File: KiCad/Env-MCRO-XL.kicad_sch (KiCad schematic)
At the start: 74 parts, among them SW1 RotaryEncoder_Switch, SW2 RotaryEncoder_Switch, SW3 RotaryEncoder_Switch, SW4 RotaryEncoder_Switch, U1 Pico

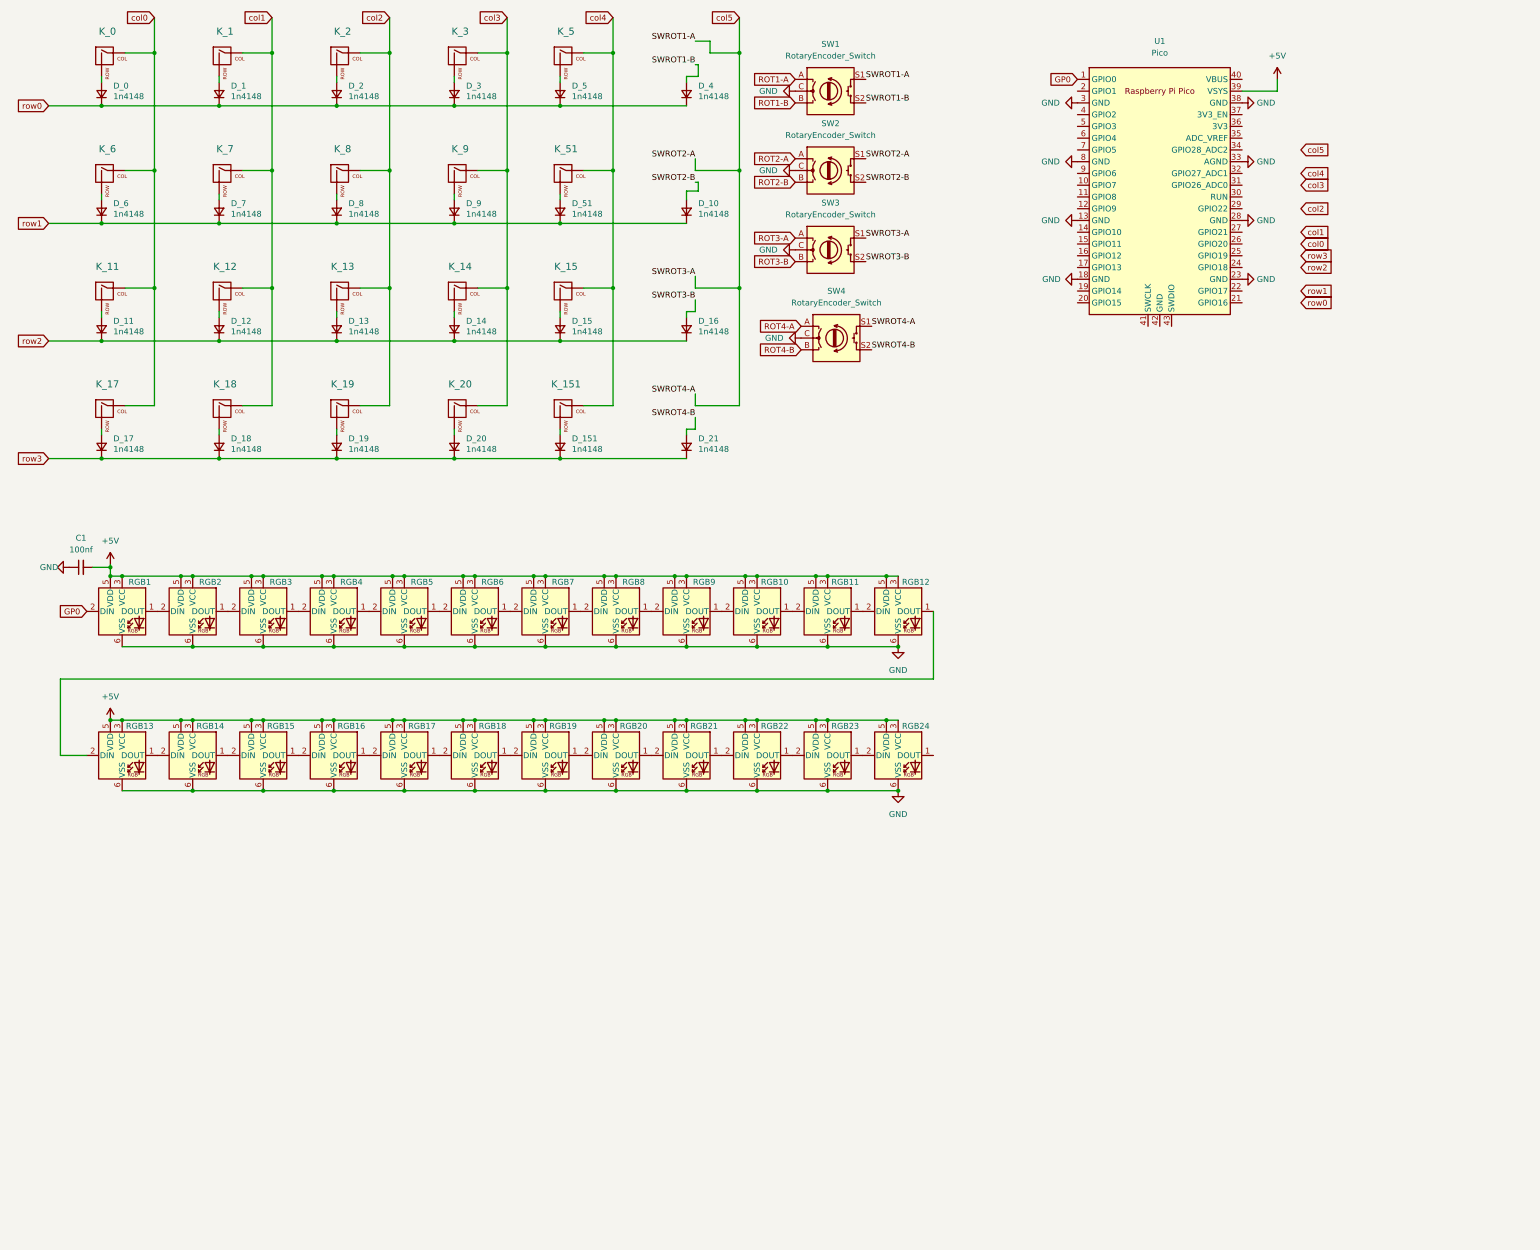
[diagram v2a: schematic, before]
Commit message: decided to revamp this project a tad.
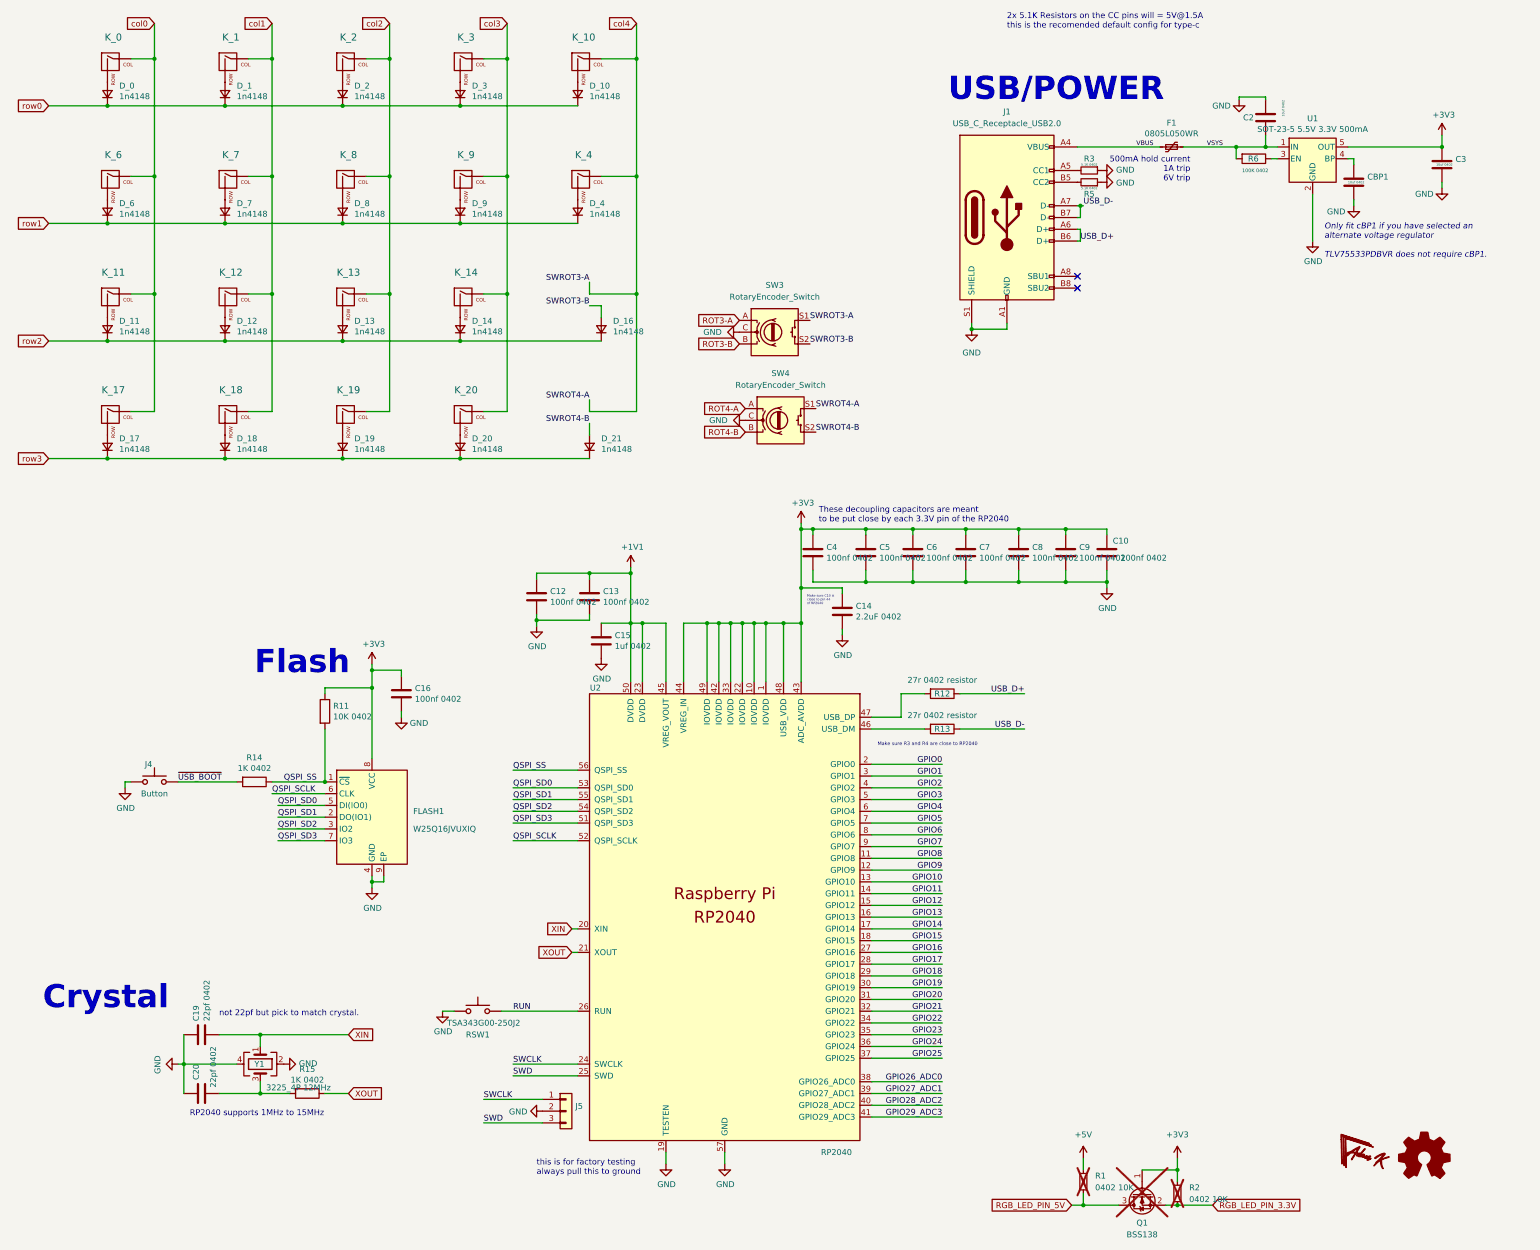
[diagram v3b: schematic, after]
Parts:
- removed C1: 100nf, Capacitor_SMD:C_0805_2012Metric, symbol Device:C_Small
- removed D_15, D_151, D_5, D_51: 1n4148, Diode_THT:D_DO-35_SOD27_P7.62mm_Horizontal, symbol Device:D_Small
- removed K_15, K_151, K_5, K_51: MX Switch, MX_Only:MXOnly-1U-NoLED, symbol MX_Alps_Hybrid:MX-NoLED
- removed RGB1, RGB10, RGB11, RGB12, RGB13, RGB14, RGB15, RGB16, RGB17, RGB18, RGB19, RGB2, RGB20, RGB21, RGB22, RGB23, RGB24, RGB3, RGB4, RGB5, RGB6, RGB7, RGB8, RGB9: WS2812, LED_SMD:LED_WS2812_PLCC6_5.0x5.0mm_P1.6mm, symbol LED:WS2812
- removed SW1, SW2: RotaryEncoder_Switch, Rotary_Encoder:RotaryEncoder_Alps_EC12E-Switch_Vertical_H20mm, symbol Device:RotaryEncoder_Switch
- removed U1: Pico, MCU_RaspberryPi_and_Boards:RPi_Pico_SMD_TH, symbol MCU_RaspberryPi_and_Boards:Pico
- added C10, C12, C13, C16, C4, C5, C6, C7, C8, C9: 100nf 0402, Capacitor_SMD:C_0402_1005Metric, symbol Device:C
- added C14: 2.2uF 0402, Capacitor_SMD:C_0402_1005Metric, symbol Device:C
- added C15: 1uf 0402, Capacitor_SMD:C_0402_1005Metric, symbol Device:C
- added C19, C20: 22pf 0402, Capacitor_SMD:C_0402_1005Metric, symbol Device:C
- added C2, C3, CBP1: 10uf 0402, Capacitor_SMD:C_0402_1005Metric, symbol Device:C
- added F1: 0805L050WR, Fuse:Fuse_0805_2012Metric, symbol Device:Polyfuse_Small
- added FLASH1: W25Q16JVUXIQ, Package_SON:Winbond_USON-8-1EP_3x2mm_P0.5mm_EP0.2x1.6mm, symbol Memory_Flash:W25Q32JVZP
- added J1: USB_C_Receptacle_USB2.0, Connector_USB:USB_C_Receptacle_HRO_TYPE-C-31-M-12, symbol Connector:USB_C_Receptacle_USB2.0
- added J4: Button, Button_Switch_SMD:SW_Push_SPST_NO_Alps_SKRK, symbol Switch:SW_Push
- added J5: Conn_01x03_Male, Connector_PinHeader_2.54mm:PinHeader_1x03_P2.54mm_Vertical, symbol Connector_Generic:Conn_01x03
- added K_10, K_4: MX Switch, MX_Only:MXOnly-1U-NoLED, symbol MX_Alps_Hybrid:MX-NoLED
- added Q1: BSS138, Package_TO_SOT_SMD:SOT-23, symbol Transistor_FET:BSS138
- added R1, R2: 0402 10K, Resistor_SMD:R_0402_1005Metric, symbol Device:R_Small
- added R11: 10K 0402, Resistor_SMD:R_0402_1005Metric, symbol Device:R
- added R12, R13: 27r 0402 resistor, Resistor_SMD:R_0402_1005Metric, symbol Device:R
- added R14, R15: 1K 0402, Resistor_SMD:R_0402_1005Metric, symbol Device:R
- added R3, R5: 5.1K 0402, Resistor_SMD:R_0402_1005Metric, symbol Device:R_Small
- added R6: 100K 0402, Resistor_SMD:R_0402_1005Metric, symbol Device:R
- added RSW1: TSA343G00-250J2, Button_Switch_SMD:SW_Push_SPST_NO_Alps_SKRK, symbol Switch:SW_Push
- added U1: SOT-23-5 5.5V 3.3V 500mA, Package_TO_SOT_SMD:SOT-23-5, symbol Regulator_Linear:AP131-15
- added U2: RP2040, RP2040_minimal:RP2040-QFN-56, symbol MCU_RaspberryPi_RP2040:RP2040
- added Y1: 3225_4P 12MHz, Crystal:Crystal_SMD_3225-4Pin_3.2x2.5mm, symbol Device:Crystal_GND24
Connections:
- net col5 is gone; now on net col4: SW3.S1, SW4.S1
- net +5V: now also R1.1
- net GND: now also C10.2, C12.2, C13.2, C14.2, C15.2, C16.2, C19.1, C2.2, C20.1, C3.2, C4.2, C5.2, C6.2, C7.2, C8.2, C9.2, CBP1.2, FLASH1.4 (GND), FLASH1.9 (EP), J1.A1 (GND), J1.A12 (GND), J1.B1 (GND), J1.B12 (GND), J1.S1 (SHIELD), J4.2, J5.2 (Pin_2), R3.1, R5.1, RSW1.1, U1.2 (GND), U2.19 (TESTEN), U2.57 (GND), Y1.2, Y1.4
- net col4: now also K_10.1 (COL), K_4.1 (COL)
- net row0: now also D_10.1 (K); no longer D_4.1 (K)
- net row1: now also D_4.1 (K); no longer D_10.1 (K)
- net SWROT1-B: no longer names the net of D_4.2 (A)
- net SWROT1-B: now also K_4.2 (ROW)
- net SWROT2-B: no longer names the net of D_10.2 (A)
- net SWROT2-B: now also K_10.2 (ROW)
- new net: C20.2, R15.2, Y1.3
- new net: J1.A5 (CC1), R3.2
- new net: J1.B5 (CC2), R5.2
- new net: CBP1.1, U1.4 (BP)
- new net: R6.1, U1.3 (EN)
- new net: R13.2, U2.46 (USB_DM)
- new net: R12.2, U2.47 (USB_DP)
- new net +1V1: C12.1, C13.1, C15.1, U2.23 (DVDD), U2.45 (VREG_VOUT), U2.50 (DVDD)
- new net +3V3: C10.1, C14.1, C16.1, C3.1, C4.1, C5.1, C6.1, C7.1, C8.1, C9.1, FLASH1.8 (VCC), Q1.1 (G), R11.1, R2.1, U1.5 (OUT), U2.1 (IOVDD), U2.10 (IOVDD), U2.22 (IOVDD), U2.33 (IOVDD), U2.42 (IOVDD), U2.43 (ADC_AVDD), U2.44 (VREG_IN), U2.48 (USB_VDD), U2.49 (IOVDD)
- new net GPIO0: U2.2 (GPIO0)
- new net GPIO1: U2.3 (GPIO1)
- new net GPIO10: U2.13 (GPIO10)
- new net GPIO11: U2.14 (GPIO11)
- new net GPIO12: U2.15 (GPIO12)
- new net GPIO13: U2.16 (GPIO13)
- new net GPIO14: U2.17 (GPIO14)
- new net GPIO15: U2.18 (GPIO15)
- new net GPIO16: U2.27 (GPIO16)
- new net GPIO17: U2.28 (GPIO17)
- new net GPIO18: U2.29 (GPIO18)
- new net GPIO19: U2.30 (GPIO19)
- new net GPIO2: U2.4 (GPIO2)
- new net GPIO20: U2.31 (GPIO20)
- new net GPIO21: U2.32 (GPIO21)
- new net GPIO22: U2.34 (GPIO22)
- new net GPIO23: U2.35 (GPIO23)
- new net GPIO24: U2.36 (GPIO24)
- new net GPIO25: U2.37 (GPIO25)
- new net GPIO26_ADC0: U2.38 (GPIO26_ADC0)
- new net GPIO27_ADC1: U2.39 (GPIO27_ADC1)
- new net GPIO28_ADC2: U2.40 (GPIO28_ADC2)
- new net GPIO29_ADC3: U2.41 (GPIO29_ADC3)
- new net GPIO3: U2.5 (GPIO3)
- new net GPIO4: U2.6 (GPIO4)
- new net GPIO5: U2.7 (GPIO5)
- new net GPIO6: U2.8 (GPIO6)
- new net GPIO7: U2.9 (GPIO7)
- new net GPIO8: U2.11 (GPIO8)
- new net GPIO9: U2.12 (GPIO9)
- new net QSPI_SCLK: FLASH1.6 (CLK), U2.52 (QSPI_SCLK)
- new net QSPI_SD0: FLASH1.5 (DI(IO0)), U2.53 (QSPI_SD0)
- new net QSPI_SD1: FLASH1.2 (DO(IO1)), U2.55 (QSPI_SD1)
- new net QSPI_SD2: FLASH1.3 (IO2), U2.54 (QSPI_SD2)
- new net QSPI_SD3: FLASH1.7 (IO3), U2.51 (QSPI_SD3)
- new net QSPI_SS: FLASH1.1 (~{CS}), R11.2, R14.1, U2.56 (QSPI_SS)
- new net RGB_LED_PIN_3.3V: Q1.2 (S), R2.2
- new net RGB_LED_PIN_5V: Q1.3 (D), R1.2
- new net RUN: RSW1.2, U2.26 (RUN)
- new net SWCLK: J5.1 (Pin_1), U2.24 (SWCLK)
- new net SWD: J5.3 (Pin_3), U2.25 (SWD)
- new net USB_D+: J1.A6 (D+), J1.B6 (D+), R12.1
- new net USB_D-: J1.A7 (D-), J1.B7 (D-), R13.1
- new net VBUS: F1.2, J1.A4 (VBUS), J1.A9 (VBUS), J1.B4 (VBUS), J1.B9 (VBUS)
- new net VSYS: C2.1, F1.1, R6.2, U1.1 (IN)
- new net XIN: C19.2, U2.20 (XIN), Y1.1
- new net XOUT: R15.1, U2.21 (XOUT)
- new net ~{USB_BOOT}: J4.1, R14.2
- no-connect marks 0 -> 2
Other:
- note added: "2x 5.1K Resistors on the CC pins will = 5V@1.5A this is the recomended default config for type-c"
- note added: "500mA hold current 1A trip 6V trip"
- note added: "Crystal"
- note added: "Flash"
- note added: "Make sure C10 is close to pin 44 of RP2040"
- note added: "Make sure R3 and R4 are close to RP2040"
- note added: "Only fit cBP1 if you have selected an alternate voltage regulator TLV75533PDBVR does not require cBP1."
- note added: "RP2040 supports 1MHz to 15MHz"
- note added: "These decoupling capacitors are meant to be put close by each 3.3V pin of the RP2040"
- note added: "USB/POWER"
- note added: "not 22pf but pick to match crystal."
- note added: "this is for factory testing always pull this to ground"
- moved on the sheet: D_0, D_1, D_11, D_12, D_13, D_14, D_16, D_17, D_18, D_19, D_2, D_20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
